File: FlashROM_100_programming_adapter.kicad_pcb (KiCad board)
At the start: 2 copper layers, 18 x 40.9 mm, 2 parts, among them J1 LH535618 Socket, U1 29F010 pins to programmer

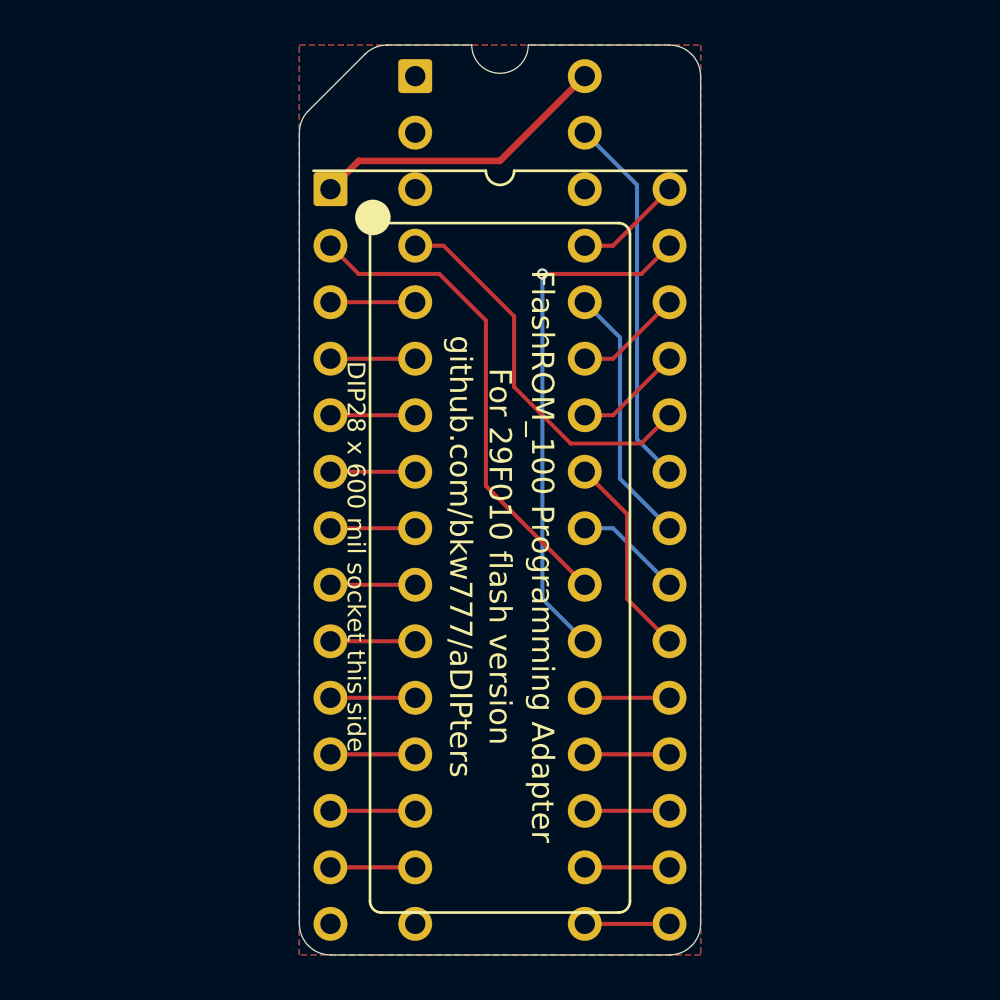
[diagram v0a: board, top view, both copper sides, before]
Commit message: various minor cleanups
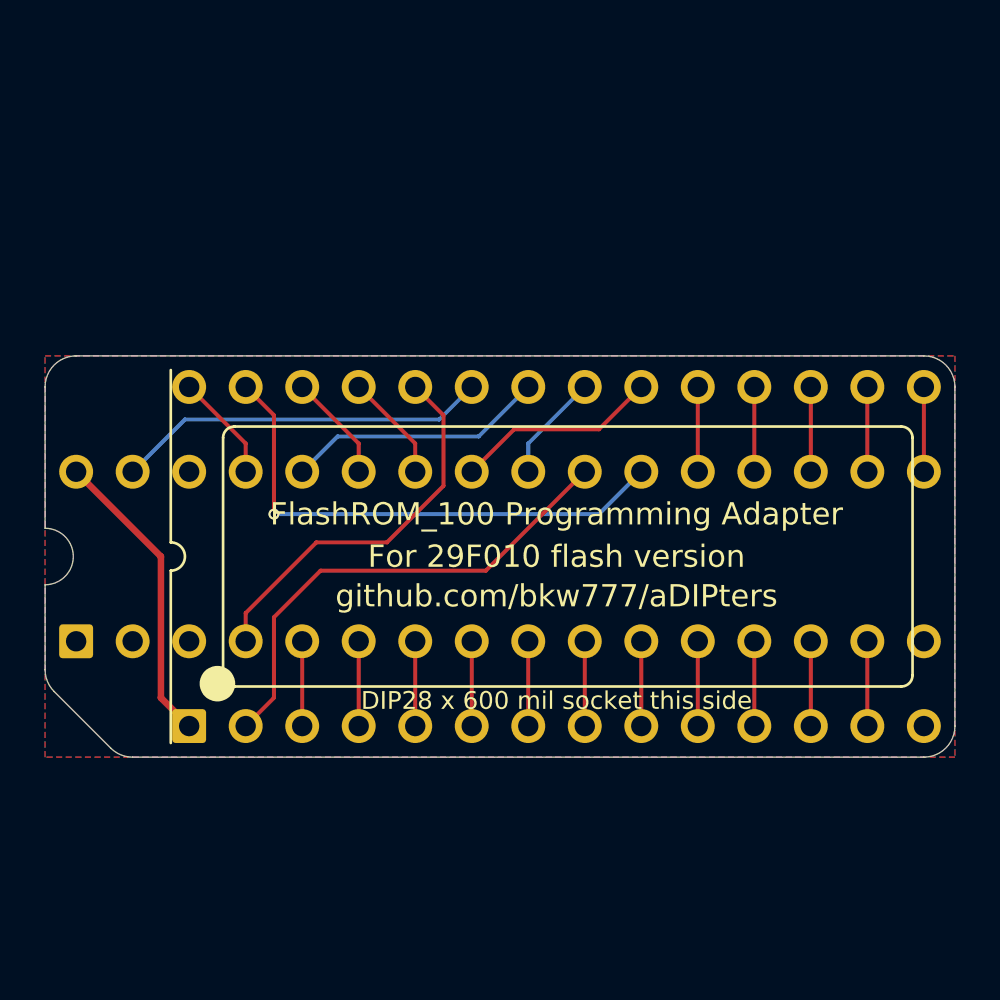
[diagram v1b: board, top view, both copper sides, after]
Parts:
- moved U1 2.54 mm to (150.0, 100.0), turned to 90 degrees
- moved J1 2.54 mm to (152.5, 100.0), turned to 90 degrees
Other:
- board size 18 x 40.9 mm -> 40.9 x 18 mm
